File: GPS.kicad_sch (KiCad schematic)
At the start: 7 parts, among them Q1 BSS138, U46 2.54mm 2x6 socket

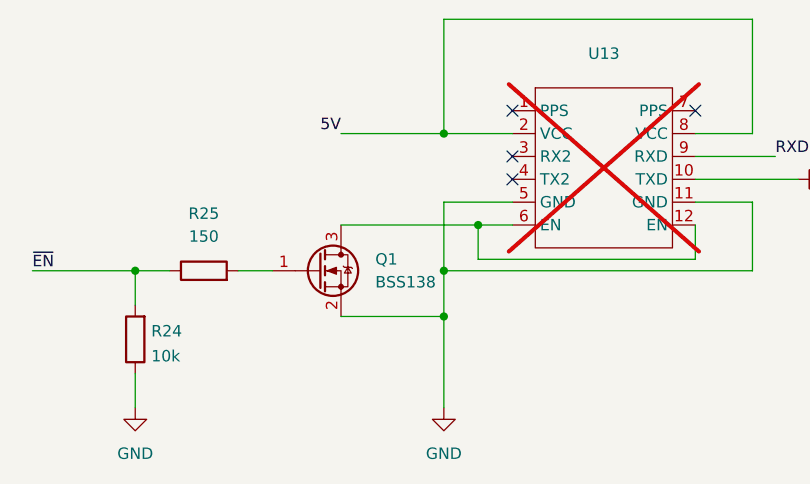
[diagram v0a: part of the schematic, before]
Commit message: Prepare v0.2
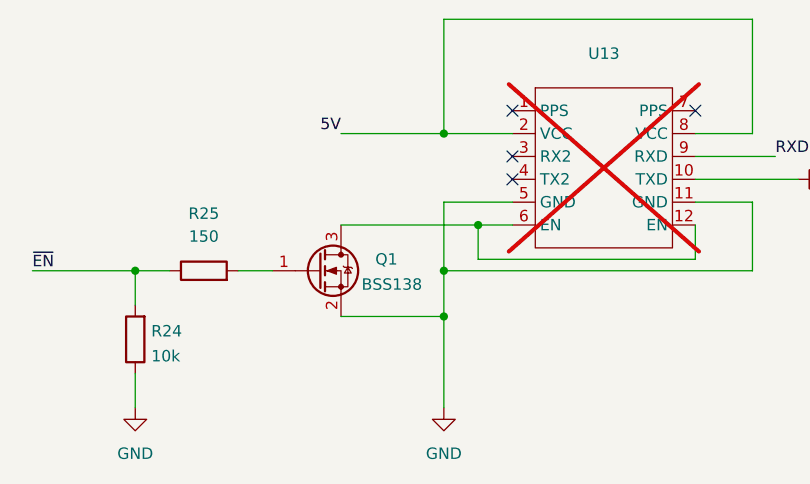
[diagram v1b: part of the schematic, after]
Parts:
- U13: footprint xtech:UM9XX_WitMotion -> local_Connectors:UM9XX_WitMotion Sabo
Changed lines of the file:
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@@
 	(title_block
 		(title "OpenMower SABO Mainboard for Series I & II")
-		(date "2025-02-26")
-		(rev "v0.1")
+		(date "2025-05-04")
+		(rev "v0.2")
 		(company "Apeheanger <joerg@ebeling.ws> for OpenMower")
 		(comment 1 "This design is licensed under CC BY-NC 4.0")
@@
 			)
 		)
-		(property "Footprint" "xtech:UM9XX_WitMotion"
+		(property "Footprint" "local_Connectors:UM9XX_WitMotion Sabo"
 			(at 184.15 107.95 0)
 			(effects
@@
 		(on_board yes)
 		(dnp no)
-		(fields_autoplaced yes)
 		(property "Reference" "Q1"
 			(at 166.37 106.6799 0)
@@
 		)
 		(property "Value" "BSS138"
-			(at 166.37 109.2199 0)
-			(effects
-				(font
+			(at 164.846 109.474 0)
+			(effects
+				(font
